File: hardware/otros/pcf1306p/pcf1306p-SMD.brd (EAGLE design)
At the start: 18.8 x 49 mm, 12 parts, among them IC23 74LS32D, IC24 74LS00D, IC25 74*157, IC26 74*157, IC3 74*157, IC4 74*157

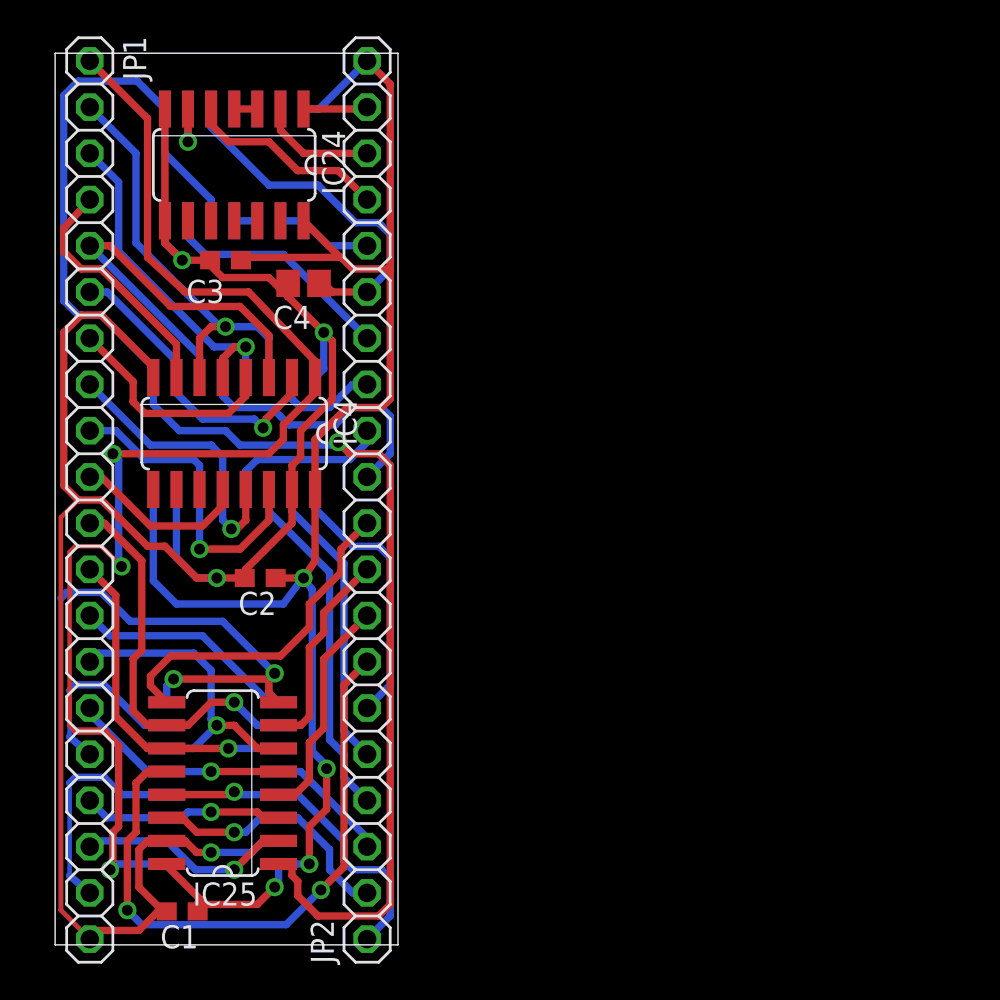
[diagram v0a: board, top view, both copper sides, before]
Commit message: Roto 90 grados el diseño
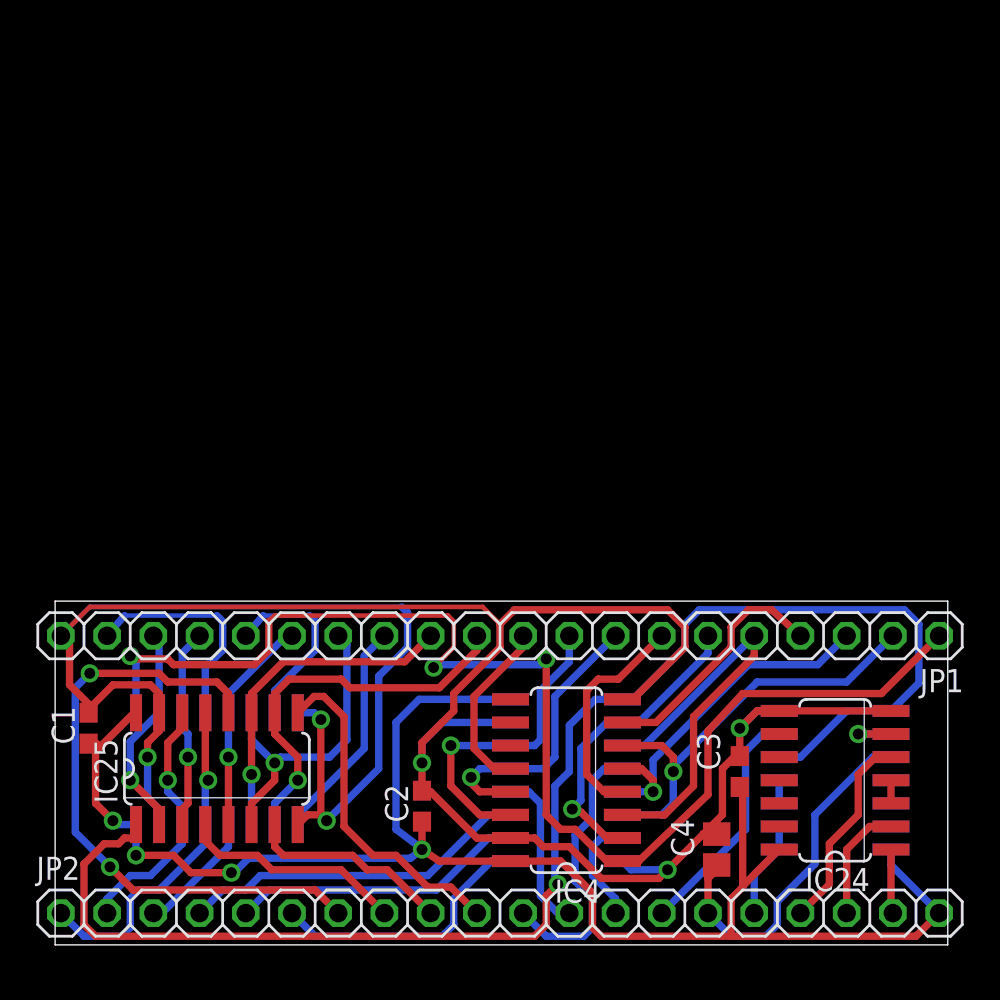
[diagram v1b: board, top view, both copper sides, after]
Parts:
- moved IC23 47.3 mm to (42.9, 9.05), turned to 90 degrees
- moved IC24 47.3 mm to (42.9, 9.05), turned to 90 degrees
- moved C3 39.9 mm to (37.6, 9.53), turned to 90 degrees
- moved C4 38.5 mm to (36.4, 5.24), turned to 90 degrees
- moved IC26 26.4 mm to (28.1, 9.05), turned to 270 degrees
- moved IC4 26.4 mm to (28.1, 9.05), turned to 90 degrees
- moved JP2 23.8 mm to (24.4, 1.75), turned to 0 degrees
- moved JP1 23.7 mm to (24.4, 17.0), turned to 180 degrees
- moved C2 15.4 mm to (20.2, 7.62), turned to 90 degrees
- moved C1 11.3 mm to (1.84, 11.9), turned to 90 degrees
- moved IC25 0.85 mm to (8.89, 9.68), turned to 0 degrees
- moved IC3 0.85 mm to (8.89, 9.68), turned to 180 degrees
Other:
- board size 18.8 x 49 mm -> 49.1 x 18.9 mm
